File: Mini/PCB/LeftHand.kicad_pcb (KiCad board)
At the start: 2 copper layers, 155.9 x 99.3 mm, 30 parts

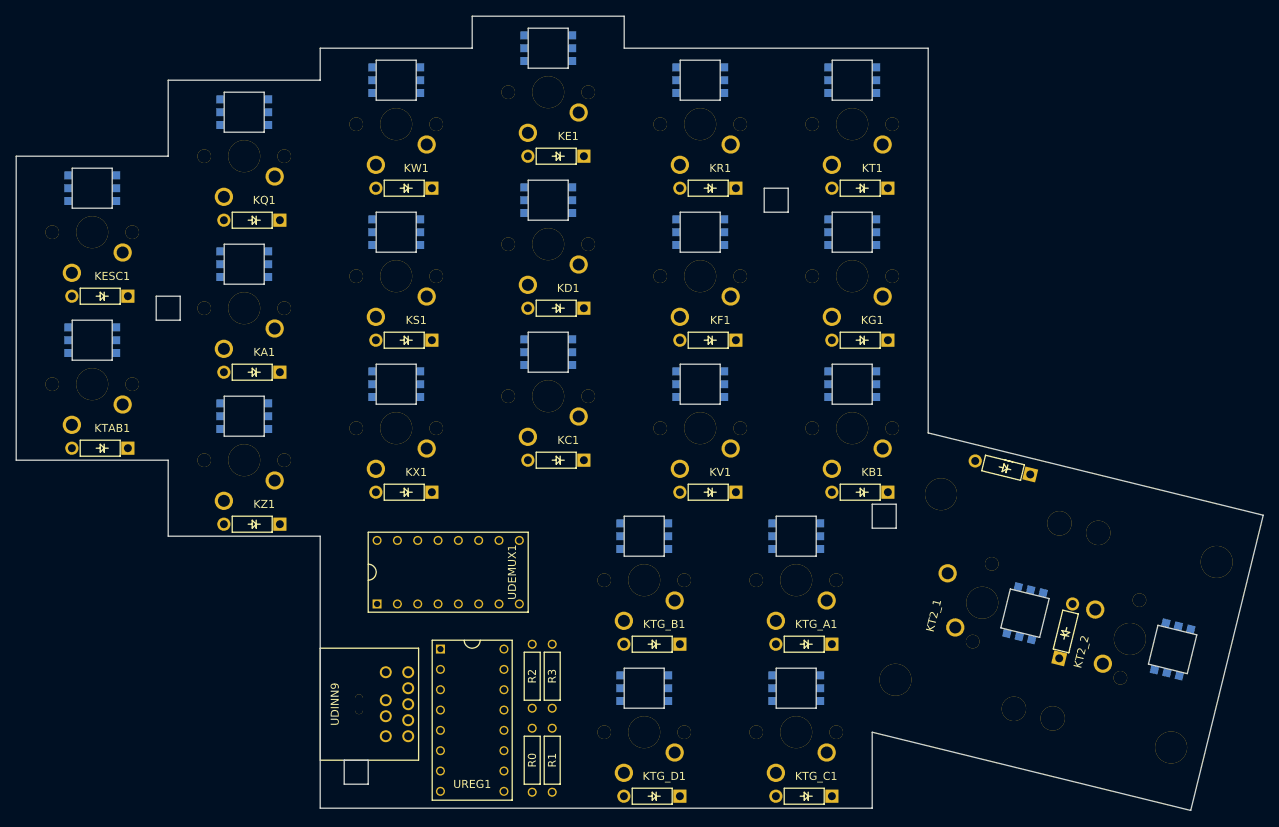
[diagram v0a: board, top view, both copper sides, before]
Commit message: Finished wiring left hand.  Generated gerber files.
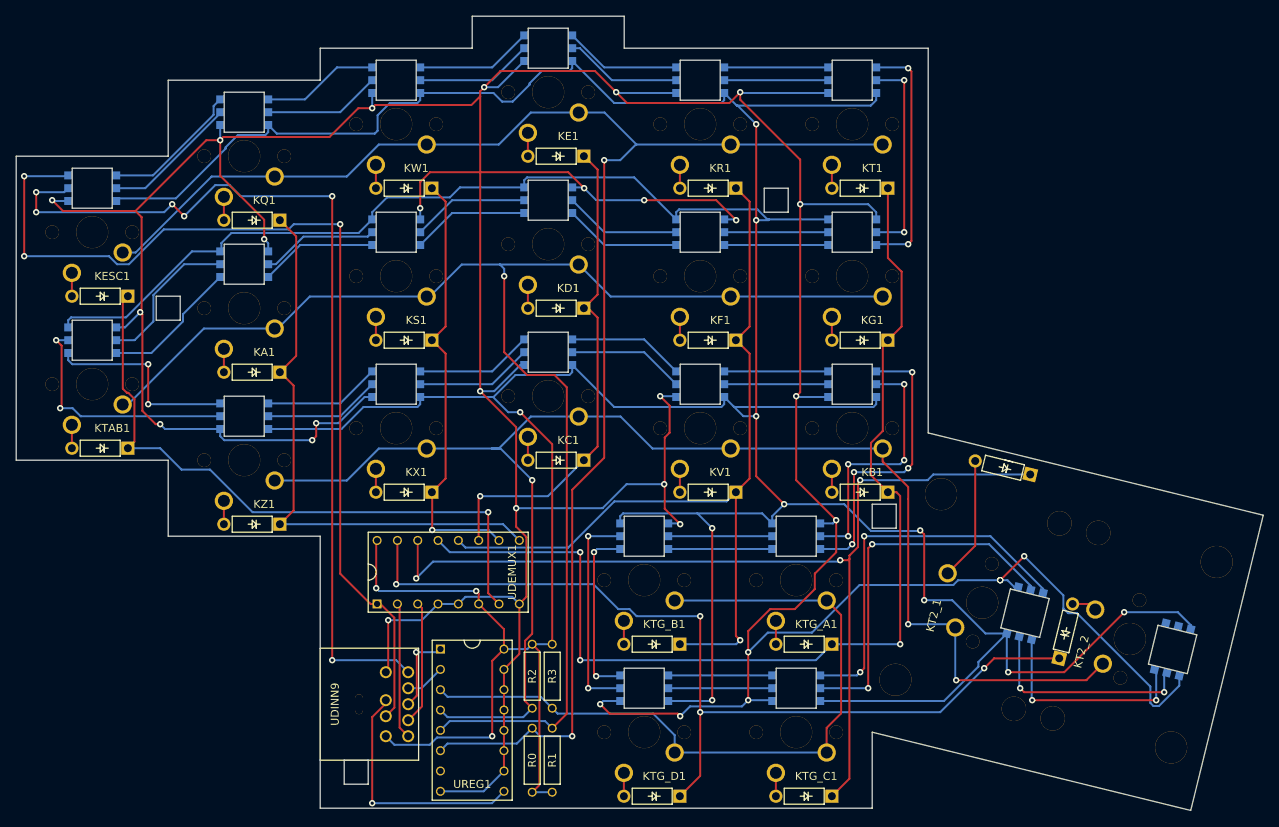
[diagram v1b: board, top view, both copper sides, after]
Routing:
- net GND: track 0.00 -> 630.8 mm, vias 0 -> 31
- net VCC: track 0.00 -> 630.8 mm, vias 0 -> 14
- net C0: track 0.00 -> 200.4 mm, vias 0 -> 2
- net C2: track 0.00 -> 184.4 mm, vias 0 -> 3
- net C1: track 0.00 -> 182.9 mm, vias 0 -> 1
- net R2: track 0.00 -> 134.2 mm, vias 0 -> 3
- net S0_DL: track 0.00 -> 123.0 mm, vias 0 -> 3
- net R1: track 0.00 -> 122.5 mm, vias 0 -> 3
- net R0: track 0.00 -> 116.4 mm, vias 0 -> 4
- net CLK_L: track 0.00 -> 115.0 mm, vias 0 -> 6
- net R3: track 0.00 -> 105.3 mm, vias 0 -> 1
- net C3: track 0.00 -> 92.3 mm
- net R7: track 0.00 -> 80.7 mm, vias 0 -> 1
- net R6: track 0.00 -> 71.9 mm
- net R4: track 0.00 -> 61.6 mm, vias 0 -> 1
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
